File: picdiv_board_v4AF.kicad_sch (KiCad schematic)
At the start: 48 parts, among them J1 DC-Input, J10 PPS_B, J11 PPS_B, J2 MountingHole_M2.5, J3 MountingHole_M2.5, J5 Conn_01x06, J6 Sync, J7 Sync, J8 10MHz, J9 10MHz, SW1 SW_DIP_x03, U1 LT1963AEST-3.3, U2 LT1963AEST-3.3, U3 PIC12F675-xSN, U5 IDT5PB1108, U6 IDT5PB1108

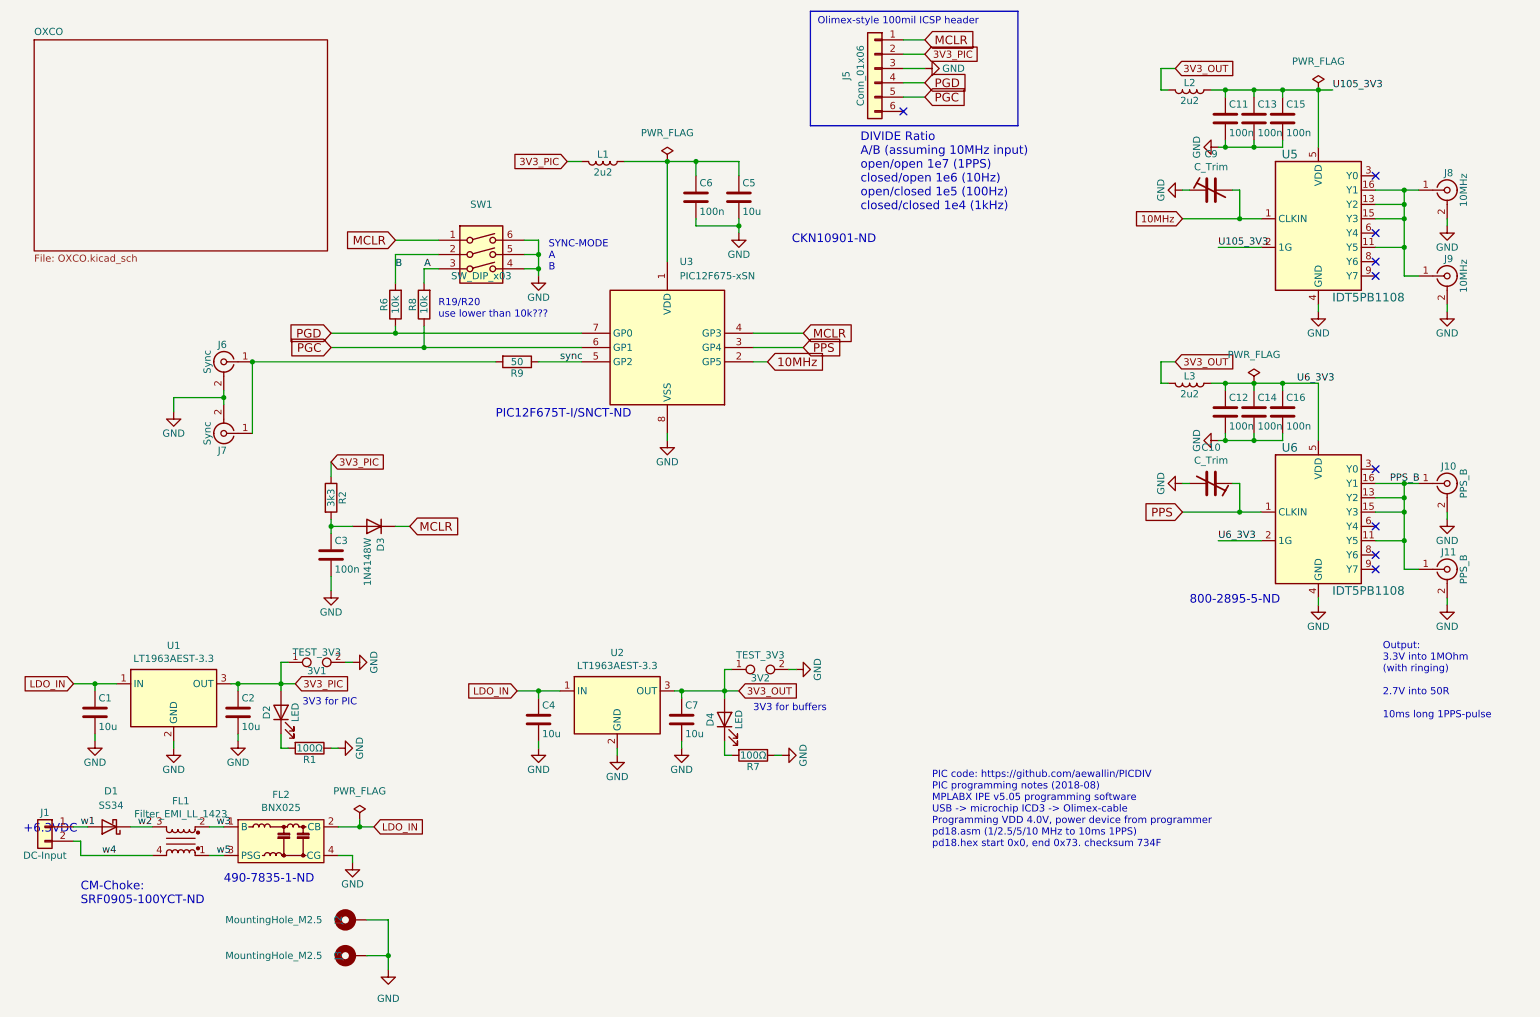
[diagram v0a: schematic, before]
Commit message: Highlight a DRC error
Needs  more work.
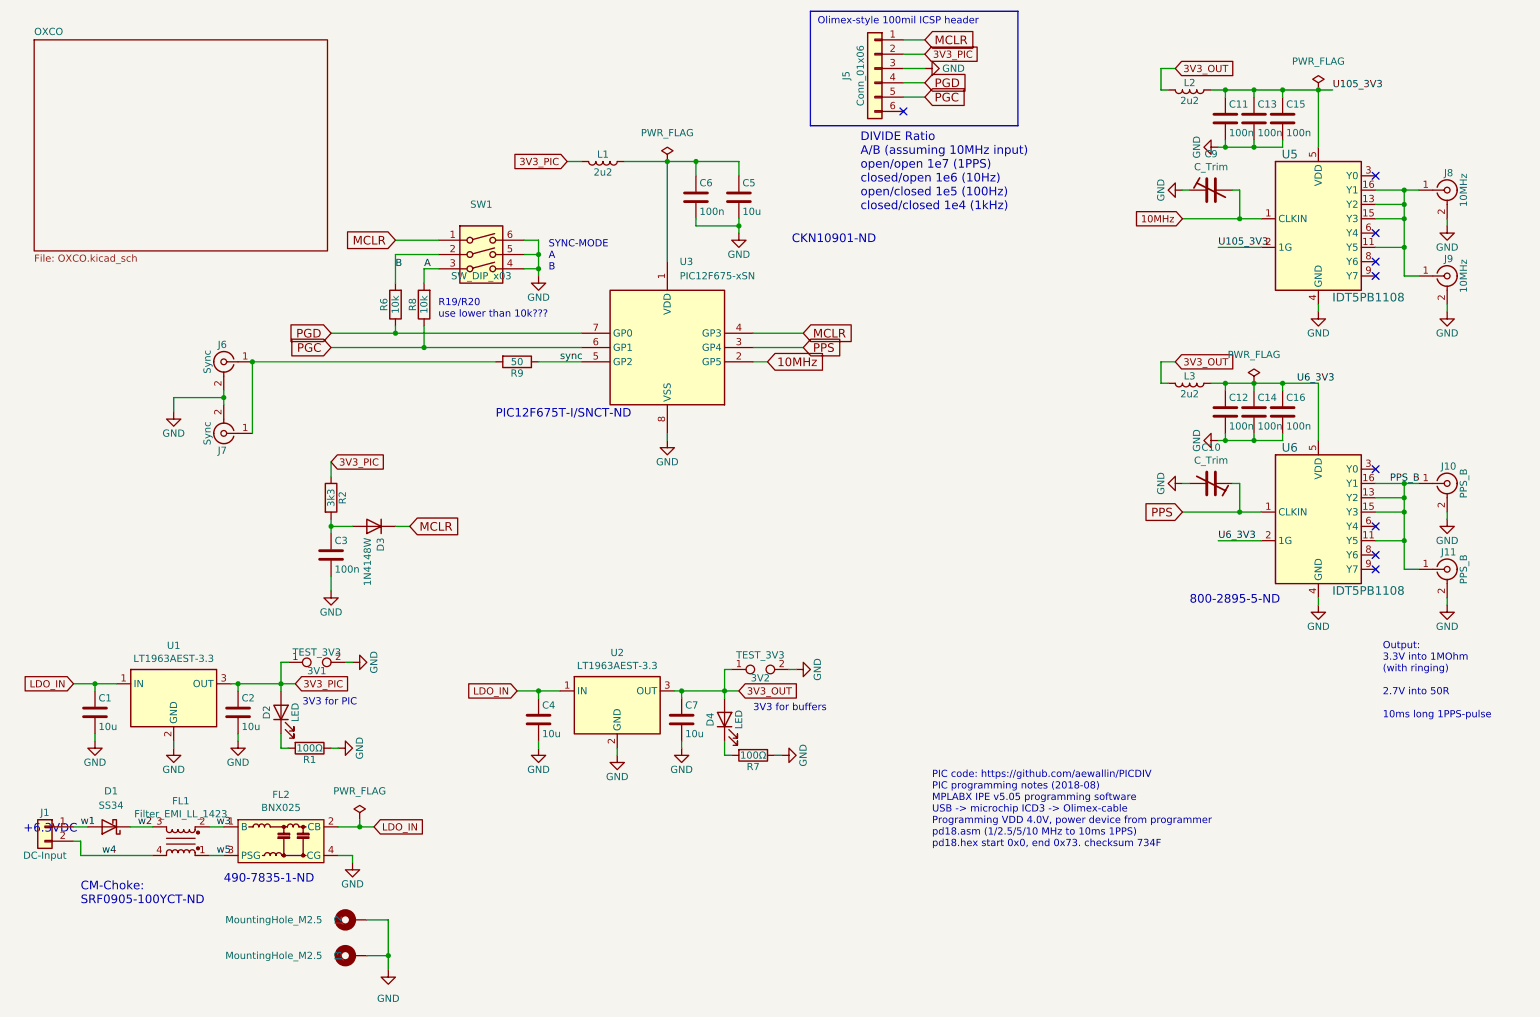
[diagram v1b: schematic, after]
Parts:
- D3: footprint Diodes_SMD:D_SOD-123 -> Diode_SMD:D_SOD-123
